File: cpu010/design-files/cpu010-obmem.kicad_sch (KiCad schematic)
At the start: 18 parts, among them U501 GAL22V10, U502 CY62158, U503 CY62158, U504 CY62158, U505 CY62158, U506 SST39SF040, U507 SST39SF040

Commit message: We have 8MB RAM now.
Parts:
- removed U501: GAL22V10, Package_DIP:DIP-24_W7.62mm_Socket, symbol jrt-ICs:GAL22V10
- added C512, C513, C514, C515, C516, C517, C518, C519: 100nF, Capacitor_SMD:C_0805_2012Metric_Pad1.18x1.45mm_HandSolder, symbol Device:C_Small
- added U501: ATF1504AS-PLCC44, Package_LCC:PLCC-44_THT-Socket, symbol jrt-ICs:ATF1504AS-PLCC44
- added U508, U509, U510, U511: CY62158, Package_SO:TSOP-II-44_10.16x18.41mm_P0.8mm, symbol jrt-Memory:CY62158
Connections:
- net A1 is gone; now on net +5V: U504.40 (CE2), U505.40 (CE2)
- net OBMEM_nA1 is gone; now on net +5V: U502.40 (CE2), U503.40 (CE2)
- net +5V: now also C512.1, C513.1, C514.1, C515.1, C516.1, C517.1, C518.1, C519.1, U501.15 (VCC), U501.23 (VCC), U501.3 (VCC), U501.35 (VCC), U508.11 (VDD), U508.33 (VDD), U508.40 (CE2), U509.11 (VDD), U509.33 (VDD), U509.40 (CE2), U510.11 (VDD), U510.33 (VDD), U510.40 (CE2), U511.11 (VDD), U511.33 (VDD), U511.40 (CE2)
- net A10: now also U508.39 (A8), U509.39 (A8), U510.39 (A8), U511.39 (A8)
- net A11: now also U508.28 (A9), U509.28 (A9), U510.28 (A9), U511.28 (A9)
- net A12: now also U508.27 (A10), U509.27 (A10), U510.27 (A10), U511.27 (A10)
- net A13: now also U508.26 (A11), U509.26 (A11), U510.26 (A11), U511.26 (A11)
- net A14: now also U508.25 (A12), U509.25 (A12), U510.25 (A12), U511.25 (A12)
- net A15: now also U508.24 (A13), U509.24 (A13), U510.24 (A13), U511.24 (A13)
- net A16: now also U508.23 (A14), U509.23 (A14), U510.23 (A14), U511.23 (A14)
- net A17: now also U508.22 (A15), U509.22 (A15), U510.22 (A15), U511.22 (A15)
- net A18: now also U508.21 (A16), U509.21 (A16), U510.21 (A16), U511.21 (A16)
- net A19: now also U508.20 (A17), U509.20 (A17), U510.20 (A17), U511.20 (A17)
- net A2: now also U508.5 (A0), U509.5 (A0), U510.5 (A0), U511.5 (A0)
- net A20: now also U508.19 (A18), U509.19 (A18), U510.19 (A18), U511.19 (A18)
- net A21: now also U508.18 (A19), U509.18 (A19), U510.18 (A19), U511.18 (A19)
- net A3: now also U508.4 (A1), U509.4 (A1), U510.4 (A1), U511.4 (A1)
- net A4: now also U508.3 (A2), U509.3 (A2), U510.3 (A2), U511.3 (A2)
- net A5: now also U508.2 (A3), U509.2 (A3), U510.2 (A3), U511.2 (A3)
- net A6: now also U508.1 (A4), U509.1 (A4), U510.1 (A4), U511.1 (A4)
- net A7: now also U508.44 (A5), U509.44 (A5), U510.44 (A5), U511.44 (A5)
- net A8: now also U508.43 (A6), U509.43 (A6), U510.43 (A6), U511.43 (A6)
- net A9: now also U508.42 (A7), U509.42 (A7), U510.42 (A7), U511.42 (A7)
- net D0: now also U509.9 (IO0), U511.9 (IO0)
- net D1: now also U509.10 (IO1), U511.10 (IO1)
- net D10: now also U508.13 (IO2), U510.13 (IO2)
- net D11: now also U508.14 (IO3), U510.14 (IO3)
- net D12: now also U508.31 (IO4), U510.31 (IO4)
- net D13: now also U508.32 (IO5), U510.32 (IO5)
- net D14: now also U508.35 (IO6), U510.35 (IO6)
- net D15: now also U508.36 (IO7), U510.36 (IO7)
- net D2: now also U509.13 (IO2), U511.13 (IO2)
- net D3: now also U509.14 (IO3), U511.14 (IO3)
- net D4: now also U509.31 (IO4), U511.31 (IO4)
- net D5: now also U509.32 (IO5), U511.32 (IO5)
- net D6: now also U509.35 (IO6), U511.35 (IO6)
- net D7: now also U509.36 (IO7), U511.36 (IO7)
- net D8: now also U508.9 (IO0), U510.9 (IO0)
- net D9: now also U508.10 (IO1), U510.10 (IO1)
- net GND: now also C512.2, C513.2, C514.2, C515.2, C516.2, C517.2, C518.2, C519.2, U501.10 (GND), U501.22 (GND), U501.30 (GND), U501.42 (GND), U508.12 (GND), U508.34 (GND), U508.6 (~{CE1}), U509.12 (GND), U509.34 (GND), U509.6 (~{CE1}), U510.12 (GND), U510.34 (GND), U510.6 (~{CE1}), U511.12 (GND), U511.34 (GND), U511.6 (~{CE1})
- net ~{RAMLR} renamed ~{RAM0LR}
- net ~{RAM0LR}: no longer U505.41 (~{OE})
- net ~{RAMLW} renamed ~{RAM0LW}
- net ~{RAM0LW}: no longer U505.17 (~{WE})
- net ~{RAMUR} renamed ~{RAM0UR}
- net ~{RAM0UR}: no longer U504.41 (~{OE})
- net ~{RAMUW} renamed ~{RAM0UW}
- net ~{RAM0UW}: no longer U504.17 (~{WE})
- new net ~{RAM2LR}: U505.41 (~{OE})
- new net ~{RAM2LW}: U505.17 (~{WE})
- new net ~{RAM2UR}: U504.41 (~{OE})
- new net ~{RAM2UW}: U504.17 (~{WE})
- new net ~{RAM4LR}: U509.41 (~{OE})
- new net ~{RAM4LW}: U509.17 (~{WE})
- new net ~{RAM4UR}: U508.41 (~{OE})
- new net ~{RAM4UW}: U508.17 (~{WE})
- new net ~{RAM6LR}: U511.41 (~{OE})
- new net ~{RAM6LW}: U511.17 (~{WE})
- new net ~{RAM6UR}: U510.41 (~{OE})
- new net ~{RAM6UW}: U510.17 (~{WE})
- no-connect marks 2 -> 0
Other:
- note added: "0-2MB"
- note added: "2-4MB"
- note added: "4-6MB"
- note added: "6-8MB"
- note removed: "Lower Word"
- note removed: "Upper word"
- moved on the sheet: C501, C502, C503, C504, C505, C506, C507, C508, C509, C510, C511, U506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

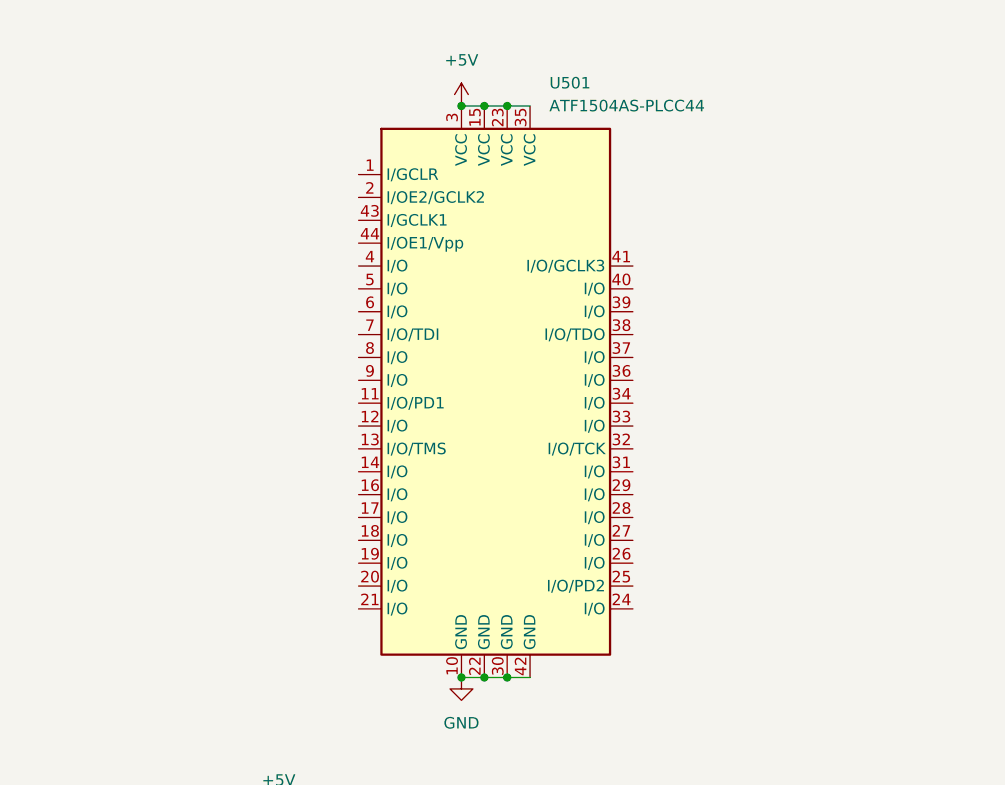
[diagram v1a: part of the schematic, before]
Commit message: Routing some I/O stuff.
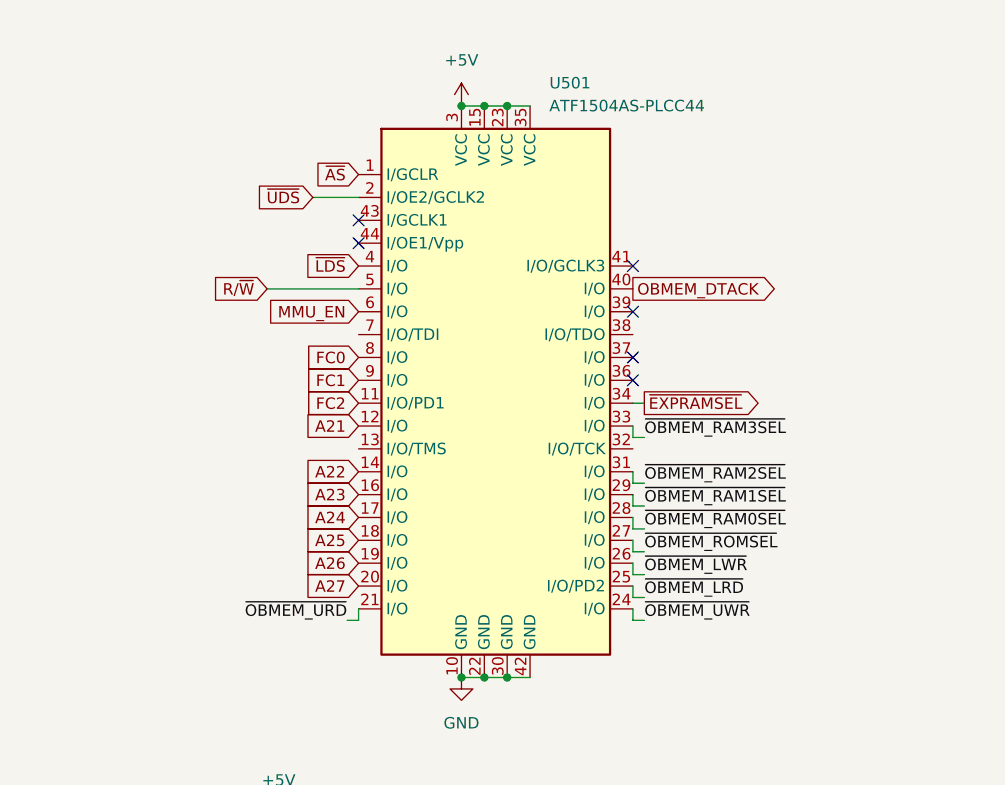
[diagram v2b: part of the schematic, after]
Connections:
- net A21: now also U501.12 (I/O)
- net ~{AS}: now reaches U501.1 (I/GCLR)
- net FC2: now reaches U501.11 (I/O/PD1)
- net A22: now reaches U501.14 (I/O)
- net A23: now reaches U501.16 (I/O)
- net A24: now reaches U501.17 (I/O)
- net A25: now reaches U501.18 (I/O)
- net A26: now reaches U501.19 (I/O)
- net ~{UDS}: now reaches U501.2 (I/OE2/GCLK2)
- net A27: now reaches U501.20 (I/O)
- net ~{OBMEM_URD}: now reaches U501.21 (I/O)
- net ~{OBMEM_UWR}: now reaches U501.24 (I/O)
- net ~{OBMEM_LRD}: now reaches U501.25 (I/O/PD2)
- net ~{OBMEM_LWR}: now reaches U501.26 (I/O)
- net ~{OBMEM_ROMSEL}: now reaches U501.27 (I/O)
- net ~{OBMEM_RAM0SEL}: now reaches U501.28 (I/O)
- net ~{OBMEM_RAM1SEL}: now reaches U501.29 (I/O)
- net ~{OBMEM_RAM2SEL}: now reaches U501.31 (I/O)
- net ~{OBMEM_RAM3SEL}: now reaches U501.33 (I/O)
- net ~{EXPRAMSEL}: now reaches U501.34 (I/O)
- net ~{LDS}: now reaches U501.4 (I/O)
- net OBMEM_DTACK: now reaches U501.40 (I/O)
- net R/~{W}: now reaches U501.5 (I/O)
- net MMU_EN: now reaches U501.6 (I/O)
- net FC0: now reaches U501.8 (I/O)
- net FC1: now reaches U501.9 (I/O)
- no-connect marks 0 -> 6
